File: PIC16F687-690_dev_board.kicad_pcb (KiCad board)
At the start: 2 copper layers, 6 parts, among them J1 Conn_01x06_Pin, U1 PIC16F690-IP

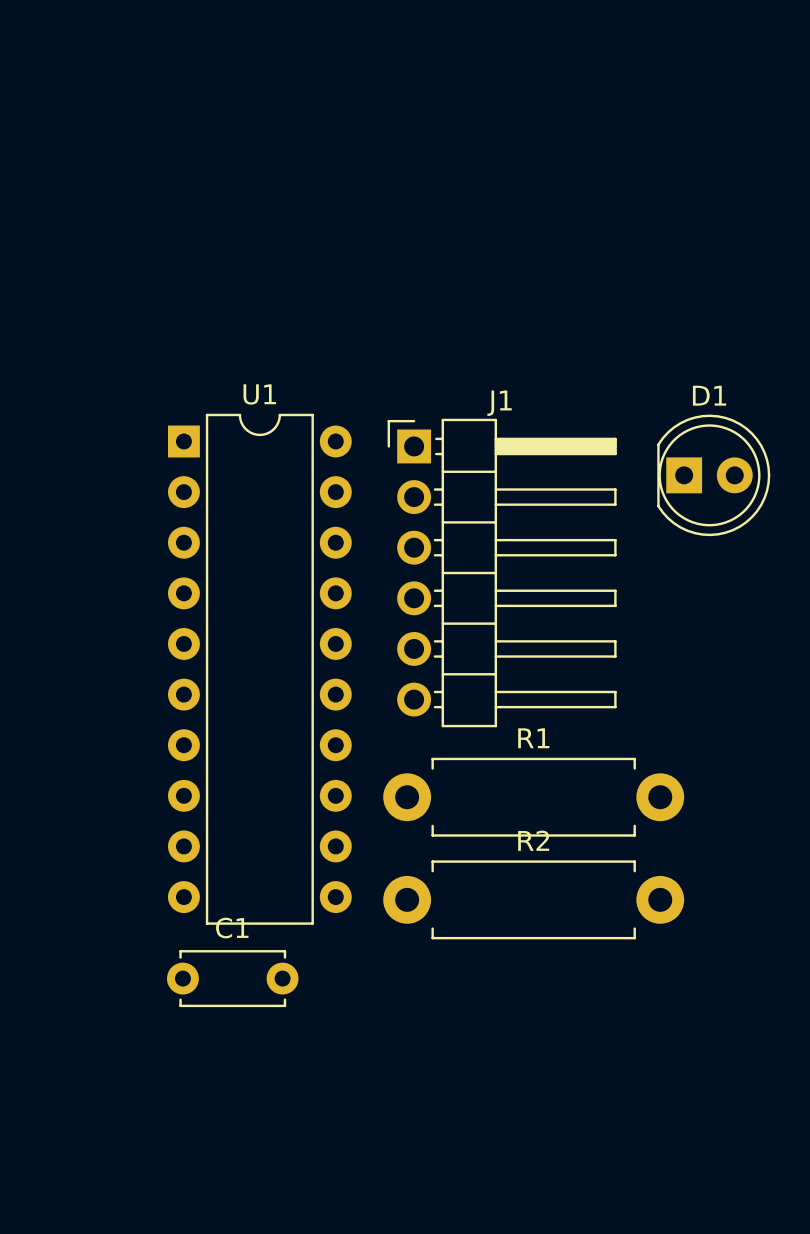
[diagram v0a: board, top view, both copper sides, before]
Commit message: finalized layout organization
finalized layout organization
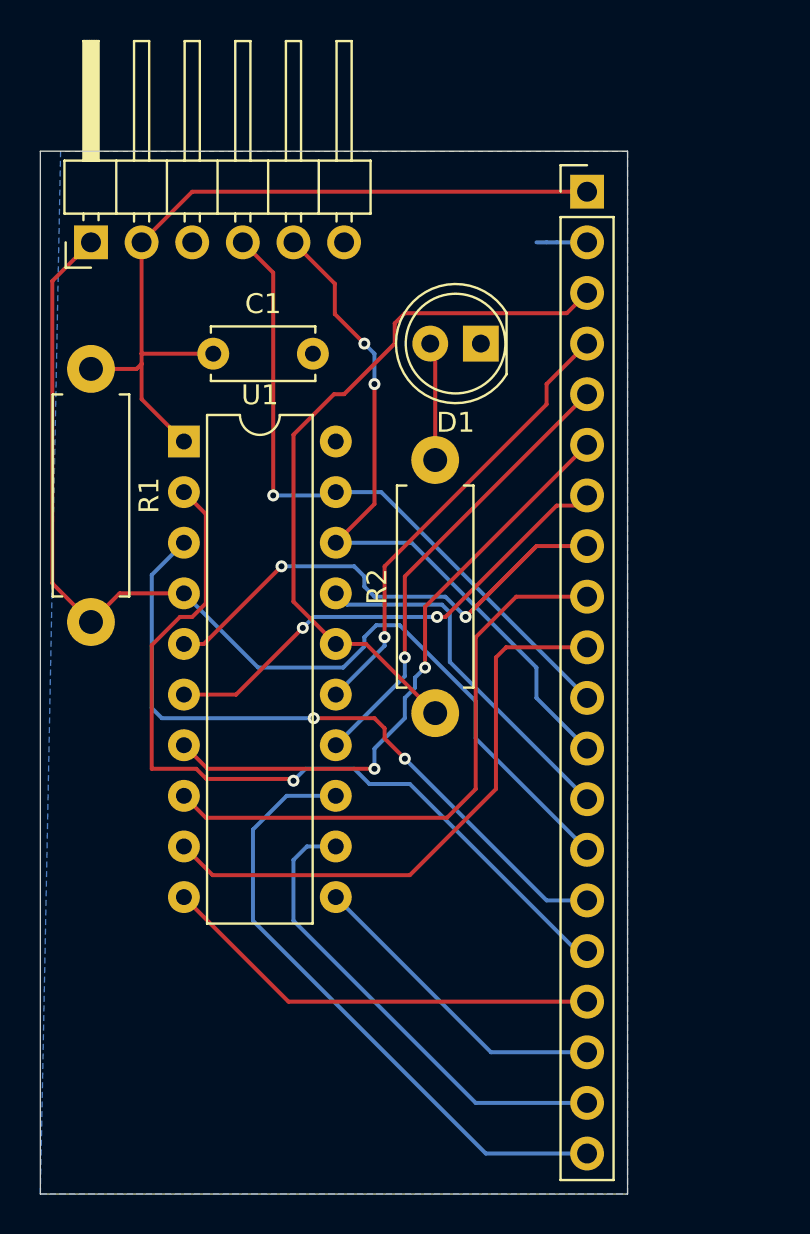
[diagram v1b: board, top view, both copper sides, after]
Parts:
- added J2: Conn_01x20_Pin, Connector_PinHeader_2.54mm:PinHeader_1x20_P2.54mm_Vertical, F.Cu at (147.8, 61.5)
- moved C1 31.4 mm to (129.1, 69.6)
- moved R1 26.7 mm to (122.9, 70.4), turned to -90 degrees
- moved J1 19.2 mm to (122.9, 64.0), turned to 90 degrees
- moved D1 12.2 mm to (142.5, 69.1), turned to 180 degrees
- moved R2 9.48 mm to (140.2, 87.6), turned to 90 degrees
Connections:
- U1 pad 10: unconnected-(U1-TX/CK/RB7-Pad10) -> Net-(J2-Pin_17)
- U1 pad 11: unconnected-(U1-SCK/SCL/RB6-Pad11) -> Net-(J2-Pin_18)
- U1 pad 12: unconnected-(U1-RX/DT/AN11/RB5-Pad12) -> Net-(J2-Pin_19)
- U1 pad 13: unconnected-(U1-SDI/SDA/AN10/RB4-Pad13) -> Net-(J2-Pin_20)
- U1 pad 14: unconnected-(U1-RC2/AN6/C12IN2-/P1D-Pad14) -> Net-(J2-Pin_5)
- U1 pad 15: unconnected-(U1-RC1/AN5/C12IN1--Pad15) -> Net-(J2-Pin_4)
- U1 pad 17: unconnected-(U1-C1OUT/T0CKI/INT/AN2/RA2-Pad17) -> Net-(J2-Pin_13)
- U1 pad 2: unconnected-(U1-T1CKI/OSC1/CLKIN/RA5-Pad2) -> Net-(J2-Pin_16)
- U1 pad 3: unconnected-(U1-~{T1G}/OSC2/CLKOUT/AN3/RA4-Pad3) -> Net-(J2-Pin_15)
- U1 pad 5: unconnected-(U1-RC5/CCP1/P1A-Pad5) -> Net-(J2-Pin_8)
- U1 pad 6: unconnected-(U1-RC4/C2OUT/P1B-Pad6) -> Net-(J2-Pin_7)
- U1 pad 7: unconnected-(U1-RC3/AN7/C12IN3-/P1C-Pad7) -> Net-(J2-Pin_6)
- U1 pad 8: unconnected-(U1-RC6/AN8/~{SS}-Pad8) -> Net-(J2-Pin_9)
- U1 pad 9: unconnected-(U1-RC7/AN9/SDO-Pad9) -> Net-(J2-Pin_10)
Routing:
- net MCLR: track 0.00 -> 54.6 mm
- net Net-(J2-Pin_16): track 0.00 -> 42.0 mm, vias 0 -> 1
- net VCC: track 0.00 -> 40.5 mm
- net Net-(J2-Pin_3): track 0.00 -> 36.1 mm
- net PGC5: track 0.00 -> 35.3 mm, vias 0 -> 2
- net Net-(J2-Pin_15): track 0.00 -> 35.1 mm, vias 0 -> 2
- net PGD4: track 0.00 -> 33.4 mm, vias 0 -> 1
- net Net-(J2-Pin_20): track 0.00 -> 31.0 mm
- net Net-(J2-Pin_6): track 0.00 -> 30.7 mm, vias 0 -> 2
- net Net-(J2-Pin_9): track 0.00 -> 29.7 mm
- net Net-(J2-Pin_8): track 0.00 -> 29.6 mm, vias 0 -> 2
- net Net-(J2-Pin_10): track 0.00 -> 29.4 mm
- net Net-(J2-Pin_7): track 0.00 -> 24.4 mm, vias 0 -> 2
- net Net-(J2-Pin_19): track 0.00 -> 24.0 mm
- net Net-(J2-Pin_4): track 0.00 -> 22.8 mm, vias 0 -> 1
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- added copper zone on B.Cu, net GND
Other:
- board outline added: 29.5 x 52.3 mm
